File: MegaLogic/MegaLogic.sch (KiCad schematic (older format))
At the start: 169 parts

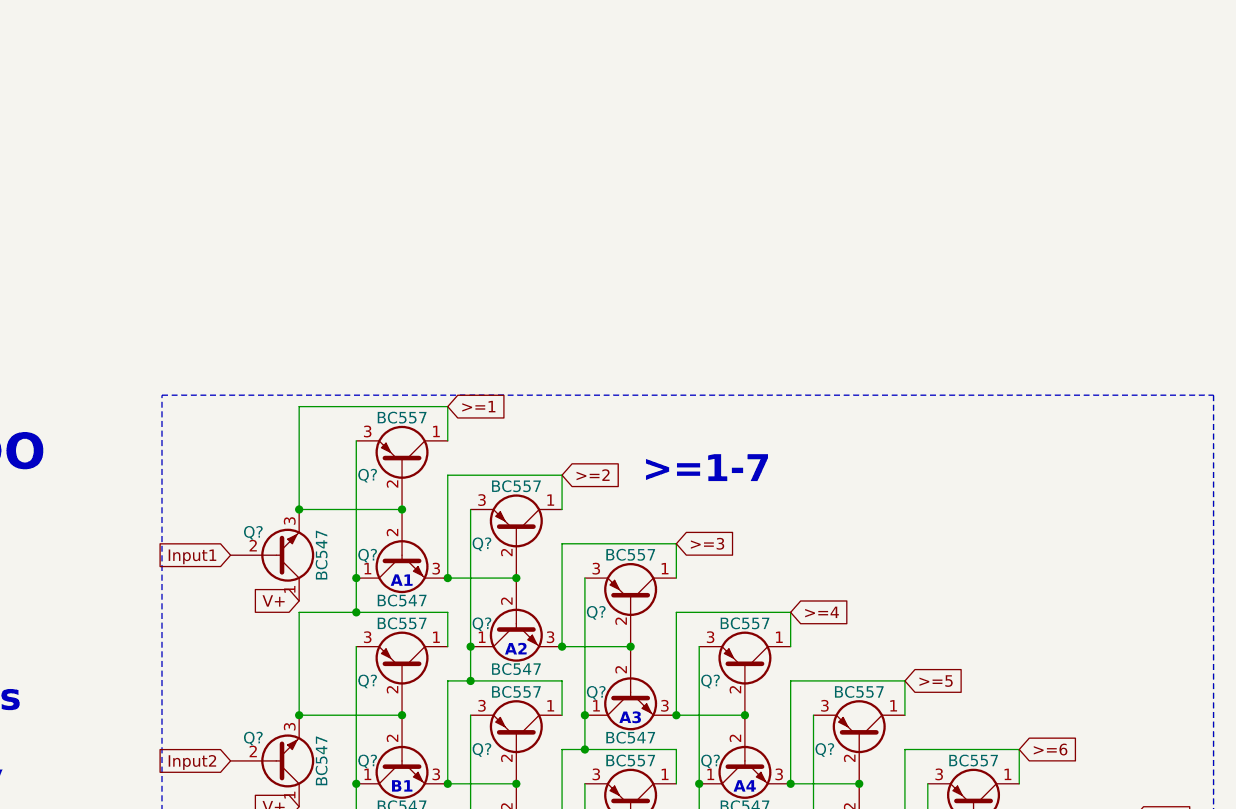
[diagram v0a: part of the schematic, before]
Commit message: Added some new ideas
Problem with 3 voice synth library
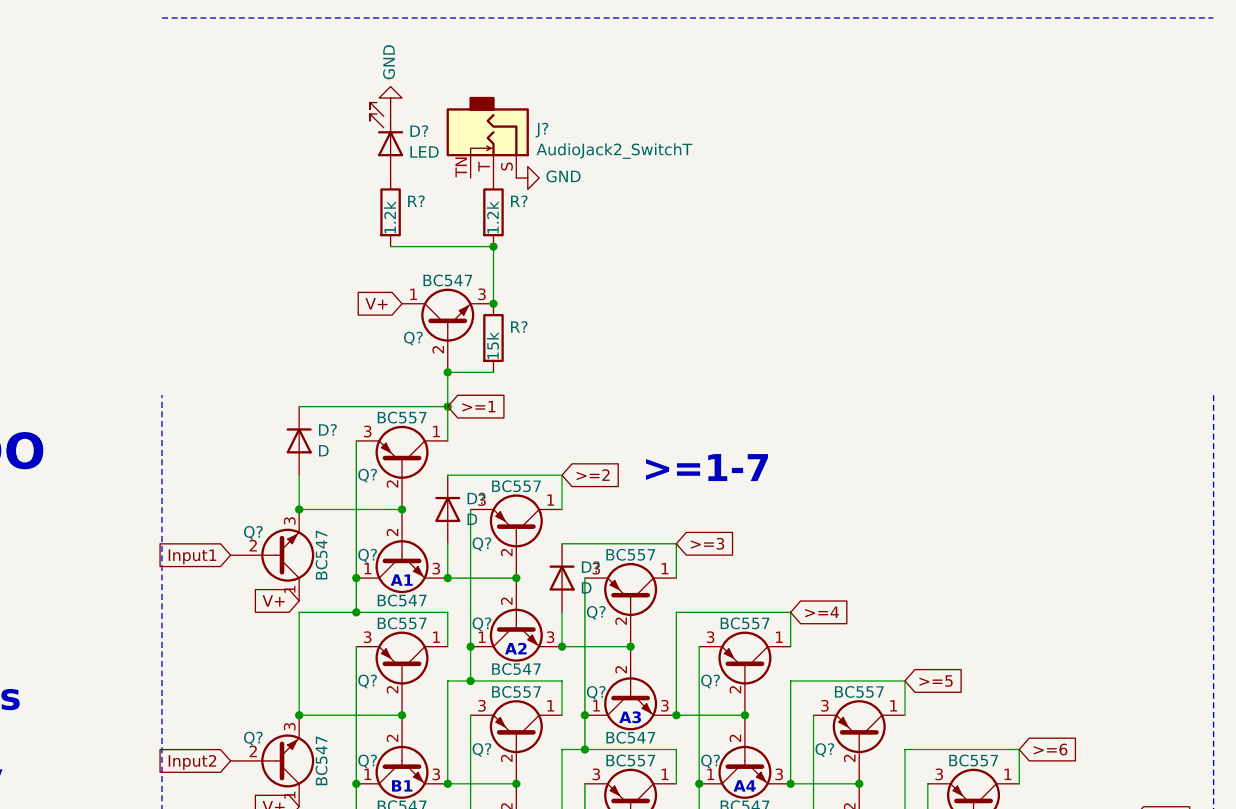
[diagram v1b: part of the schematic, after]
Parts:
- added D?: LED, symbol Device:LED
- added D? (x3): D, symbol Device:D
- added J?: AudioJack2_SwitchT, symbol Connector:AudioJack2_SwitchT
- added Q?: BC547, Package_TO_SOT_THT:TO-92_Inline, symbol Transistor_BJT:BC547
- added R?: 15k, symbol Device:R
- added R? (x2): 1.2k, symbol Device:R
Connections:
- net >=1: now also D?.1 (K), Q?.2 (B), R?.2; no longer Q?.2 (B), Q?.2 (B), Q?.3 (E)
- net >=2: now also D?.1 (K); no longer Q?.2 (B), Q?.2 (B), Q?.3 (E)
- net >=3: now also D?.1 (K); no longer Q?.2 (B), Q?.2 (B), Q?.3 (E)
- net GND: now also D?.1 (K), J?.S
- net V+: now also Q?.1 (C)
- new net: D?.2 (A), Q?.2 (B), Q?.2 (B), Q?.3 (E) (x3)
- new net: J?.T, R?.1
- new net: D?.2 (A), R?.1
- new net: Q?.3 (E), R?.1, R?.2, R?.2
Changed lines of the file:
@@
 $EndComp
-Wire Wire Line
-	13000 750  13000 1200
 Wire Wire Line
 	13500 900  13500 750
@@
 Wire Wire Line
 	13000 1200 13300 1200
-Connection ~ 13000 1200
 Connection ~ 13300 1200
 Text Notes 12750 1250 0    50   ~ 10
@@
 	13000 600  13000 450
 Wire Wire Line
-	12350 900  12350 450
-Wire Wire Line
 	12350 450  13000 450
-Connection ~ 12350 900
-Wire Wire Line
-	13500 1500 13500 1050
 Wire Wire Line
 	13500 1050 14000 1050
@@
 Wire Wire Line
 	13500 1500 13800 1500
-Connection ~ 13500 1500
 Connection ~ 13800 1500
 Wire Wire Line
@@
 Connection ~ 15100 2850
 Wire Notes Line
-	11750 400  16350 400
+	11750 -1250 16350 -1250
 Wire Notes Line
 	16350 400  16350 7300
@@
 Connection ~ -2850 3300
 Connection ~ -2750 2850
+$Comp
+L Connector:AudioJack2_SwitchT J?
+U 1 1 5F6FE61C
+P 13200 -750
+F 0 "J?" V 13186 -562 50  0000 L CNN
+F 1 "AudioJack2_SwitchT" V 13277 -562 50  0000 L CNN
+F 2 "" H 13200 -750 50  0001 C CNN
+F 3 "~" H 13200 -750 50  0001 C CNN
+	1    13200 -750
+	0    1    1    0
+$EndComp
+$Comp
+L Device:LED D?
+U 1 1 5F75F938
+P 12750 -700
+F 0 "D?" V 12697 -620 50  0000 L CNN
+F 1 "LED" V 12788 -620 50  0000 L CNN
+F 2 "" H 12750 -700 50  0001 C CNN
+F 3 "~" H 12750 -700 50  0001 C CNN
+	1    12750 -700
+	0    1    1    0
+$EndComp
+$Comp
+L Transistor_BJT:BC547 Q?
+U 1 1 5F7C7DD5
+P 13000 100
+F 0 "Q?" V 12950 250 50  0000 C CNN
+F 1 "BC547" V 13200 100 50  0000 C CNN
+F 2 "Package_TO_SOT_THT:TO-92_Inline" H 13200 25  50  0001 L CIN
+F 3 "http://www.fairchildsemi.com/ds/BC/BC547.pdf" H 13000 100 50  0001 L CNN
+	1    13000 100
+	0    -1   -1   0
+$EndComp
+$Comp
+L Device:R R?
+U 1 1 5F8578AF
+P 13200 150
+F 0 "R?" H 13270 196 50  0000 L CNN
+F 1 "15k" V 13200 50  50  0000 L CNN
+F 2 "" V 13130 150 50  0001 C CNN
+F 3 "~" H 13200 150 50  0001 C CNN
+	1    13200 150
+	1    0    0    -1
+$EndComp
+$Comp
+L Device:R R?
+U 1 1 5F91CAF6
+P 12750 -400
+F 0 "R?" H 12820 -354 50  0000 L CNN
+F 1 "1.2k" V 12750 -500 50  0000 L CNN
+F 2 "" V 12680 -400 50  0001 C CNN
+F 3 "~" H 12750 -400 50  0001 C CNN
+	1    12750 -400
+	1    0    0    -1
+$EndComp
+$Comp
+L Device:R R?
+U 1 1 5F94D7F7
+P 13200 -400
+F 0 "R?" H 13270 -354 50  0000 L CNN
+F 1 "1.2k" V 13200 -500 50  0000 L CNN
+F 2 "" V 13130 -400 50  0001 C CNN
+F 3 "~" H 13200 -400 50  0001 C CNN
+	1    13200 -400
+	1    0    0    -1
+$EndComp
+Wire Wire Line
+	13200 0    13200 -250
+Wire Wire Line
+	13200 -250 12750 -250
+Connection ~ 13200 -250
+Connection ~ 13200 0
+Wire Wire Line
+	13200 300  13000 300
+Wire Wire Line
+	13000 300  13000 450
+Connection ~ 13000 300
+Connection ~ 13000 450
+Text GLabel 12800 0    0    50   Input ~ 0
+V+
+$Comp
+L power:GND #PWR?
+U 1 1 5FB987E7
+P 13300 -550
+F 0 "#PWR?" H 13300 -800 50  0001 C CNN
+F 1 "GND" V 13305 -678 50  0000 R CNN
+F 2 "" H 13300 -550 50  0001 C CNN
+F 3 "" H 13300 -550 50  0001 C CNN
+	1    13300 -550
+	0    -1   -1   0
+$EndComp
+$Comp
+L power:GND #PWR?
+U 1 1 5FB9BF51
+P 12750 -850
+F 0 "#PWR?" H 12750 -1100 50  0001 C CNN
+F 1 "GND" V 12755 -978 50  0000 R CNN
+F 2 "" H 12750 -850 50  0001 C CNN
+F 3 "" H 12750 -850 50  0001 C CNN
+	1    12750 -850
+	-1   0    0    1
+$EndComp
+$Comp
+L Device:D D?
+U 1 1 5FBFD367
+P 12350 600
+F 0 "D?" V 12304 680 50  0000 L CNN
+F 1 "D" V 12395 680 50  0000 L CNN
+F 2 "" H 12350 600 50  0001 C CNN
+F 3 "~" H 12350 600 50  0001 C CNN
+	1    12350 600
+	0    1    1    0
+$EndComp
+Wire Wire Line
+	12350 900  12350 750
+Connection ~ 12350 900
+$Comp
+L Device:D D?
+U 1 1 5FC93CF3
+P 13000 900
+F 0 "D?" V 12954 980 50  0000 L CNN
+F 1 "D" V 13045 980 50  0000 L CNN
+F 2 "" H 13000 900 50  0001 C CNN
+F 3 "~" H 13000 900 50  0001 C CNN
+	1    13000 900
+	0    1    1    0
+$EndComp
+Wire Wire Line
+	13000 1050 13000 1200
+Connection ~ 13000 1200
+$Comp
+L Device:D D?
+U 1 1 5FCF6EE0
+P 13500 1200
+F 0 "D?" V 13454 1280 50  0000 L CNN
+F 1 "D" V 13545 1280 50  0000 L CNN
+F 2 "" H 13500 1200 50  0001 C CNN
+F 3 "~" H 13500 1200 50  0001 C CNN
+	1    13500 1200
+	0    1    1    0
+$EndComp
+Wire Wire Line
+	13500 1350 13500 1500
+Connection ~ 13500 1500
 $EndSCHEMATC
